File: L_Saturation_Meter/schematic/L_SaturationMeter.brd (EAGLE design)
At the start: 130 x 60 mm, 77 parts, among them IC1 LM317, IC4 LM358, SW1 DUR_10X, T1 IRF830, T2 BC847, T3 BC847, T4 BC847, T5 BC847, T6 IRF830, T7 IRF830, X1 I_SENSE_100x, X2 POWER_12V, X3 L_TEST_END, X4 I_SENSE_10x, X5 Synchro, X6 L_TEST_END

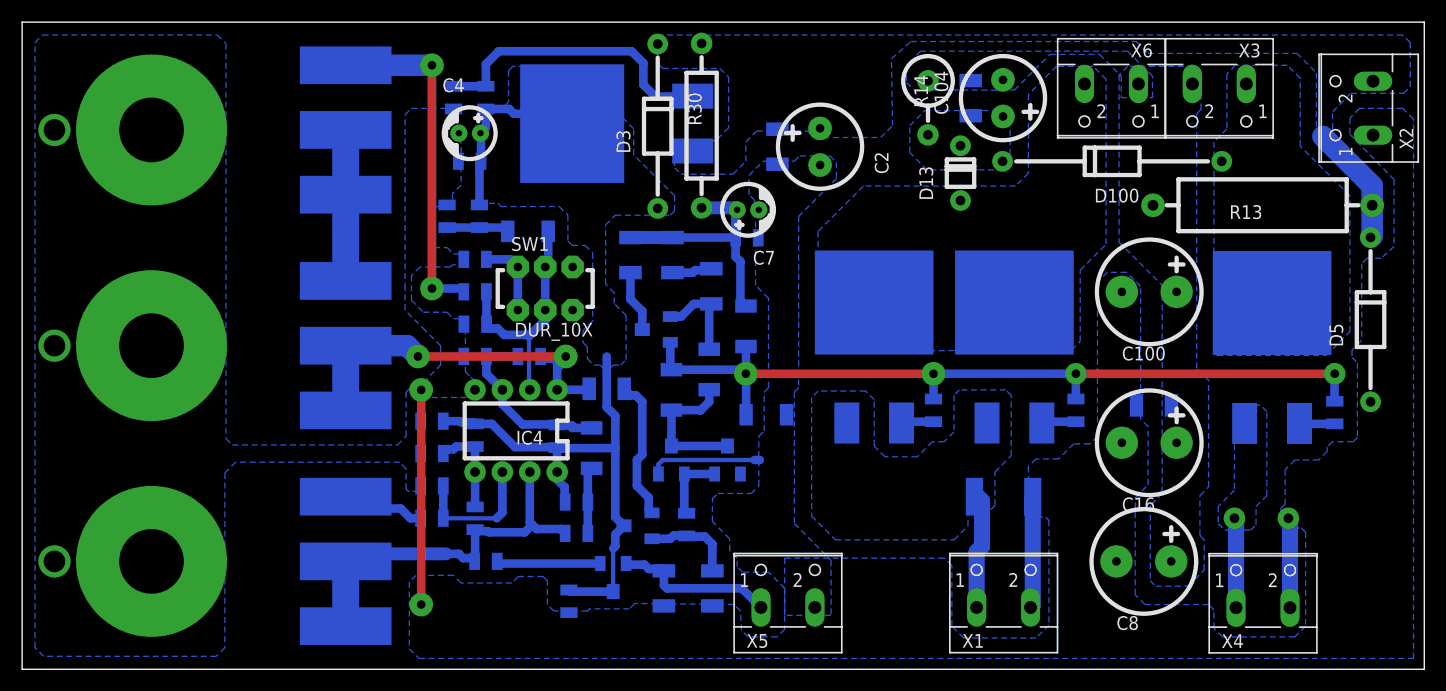
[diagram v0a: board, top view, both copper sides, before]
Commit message: L saturation meter. Routed
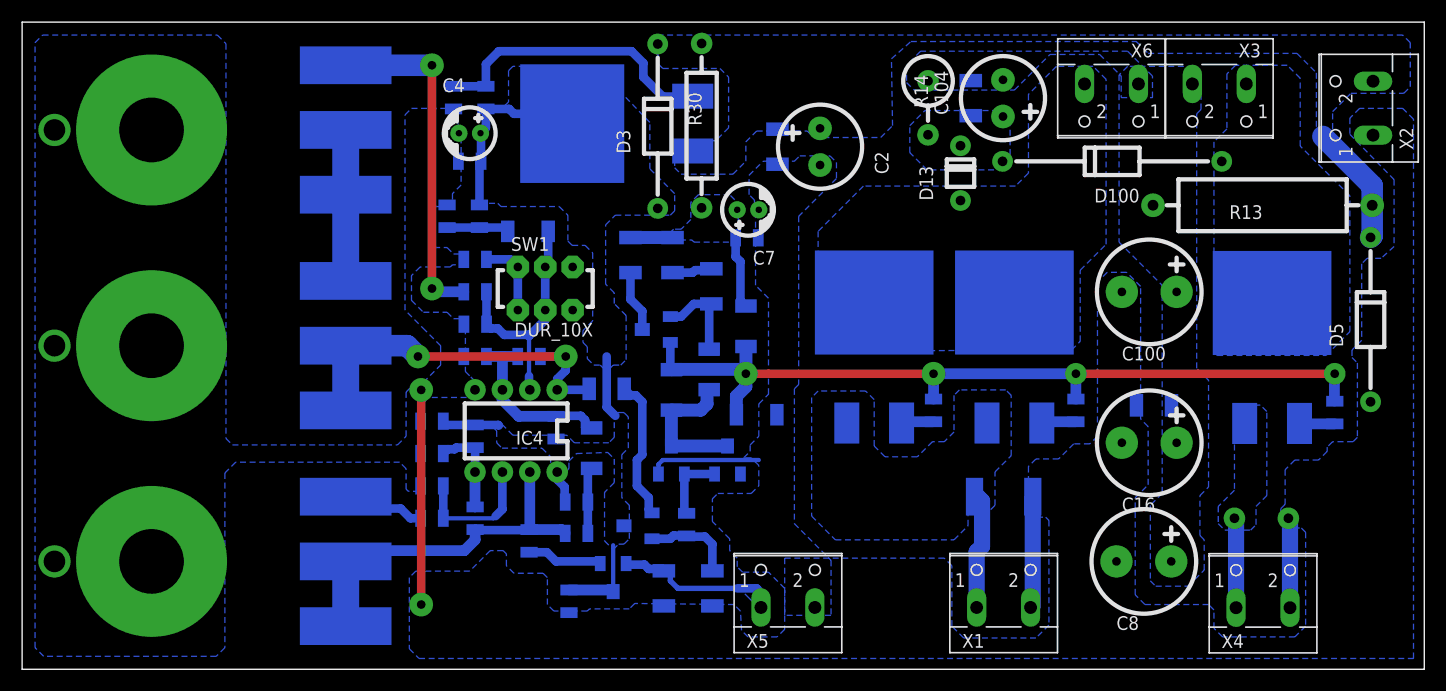
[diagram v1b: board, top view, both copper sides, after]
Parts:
- moved R18 4.43 mm to (47.0, 11.9), turned to 90 degrees
- moved D14 0.90 mm to (68.1, 23.6)
- moved R3 0.81 mm to (49.5, 22.4)
- moved R16 0.10 mm to (42.0, 21.6)
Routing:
- net +VCC: track 67.1 -> 40.7 mm
- net N$33: track 22.5 -> 10.6 mm
- net N$19: track 9.63 -> 7.03 mm
- net N$13: track 35.6 -> 33.7 mm
- net N$20: track 15.0 -> 14.2 mm
- net N$14: track 17.3 -> 16.8 mm
- added copper zone on layer 16, net N$20
- added copper zone on layer 16, net N$33

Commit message: L saturation meter. tiny fixes
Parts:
- R1: value 1K0 -> 5K6
- R19: value 510R -> 470R
- R2: value 3K0 -> 1K0
- R24: value 330R -> 470R

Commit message: L saturation meter. Final changes
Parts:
- R1: value 5K6 -> 4K7
- R13: value 1R0 -> 1R5
- R25, R26: value 510R -> 240R
- R27: value 20R -> 10R
- R6: value 1K0 -> 4K7
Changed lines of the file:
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@@
 <layer number="14" name="Route14" color="1" fill="6" visible="no" active="no"/>
 <layer number="15" name="Route15" color="4" fill="6" visible="no" active="no"/>
-<layer number="16" name="Bottom" color="1" fill="1" visible="no" active="yes"/>
+<layer number="16" name="Bottom" color="1" fill="1" visible="yes" active="yes"/>
 <layer number="17" name="Pads" color="2" fill="1" visible="yes" active="yes"/>
 <layer number="18" name="Vias" color="2" fill="1" visible="no" active="yes"/>
@@
 <attribute name="VALUE" x="71.69" y="26" size="1.27" layer="28" font="vector" ratio="20" rot="MR90"/>
 </element>
-<element name="R13" library="__MyCommonLib1" package="R_2.0W" value="1R0" x="115.01" y="43.02" smashed="yes" rot="R180">
+<element name="R13" library="__MyCommonLib1" package="R_2.0W" value="1R5" x="115.01" y="43.02" smashed="yes" rot="R180">
 <attribute name="NAME" x="115.01" y="43.02" size="1.27" layer="25" font="vector" ratio="20" rot="R180"/>
 <attribute name="VALUE" x="115.01" y="43.02" size="1.27" layer="27" font="vector" ratio="20" rot="R180"/>
@@
 <attribute name="VALUE" x="57.66" y="47.81" size="1.27" layer="27" font="vector" ratio="20" rot="R90"/>
 </element>
-<element name="R1" library="__MyCommonLib1" package="RSMD_0805" value="5K6" x="40" y="53" smashed="yes" rot="MR90">
+<element name="R1" library="__MyCommonLib1" package="RSMD_0805" value="4K7" x="40" y="53" smashed="yes" rot="MR90">
 <attribute name="NAME" x="40" y="53" size="1.27" layer="26" font="vector" ratio="20" rot="MR90"/>
 <attribute name="VALUE" x="36.9" y="51.3" size="1.27" layer="28" font="vector" ratio="20" rot="MR90"/>
@@
 <attribute name="VALUE" x="54.5" y="16.9" size="1.27" layer="28" font="vector" ratio="20" rot="MR90"/>
 </element>
-<element name="R6" library="__MyCommonLib1" package="RSMD_0805" value="1K0" x="51.4" y="15.5" smashed="yes" rot="MR180">
+<element name="R6" library="__MyCommonLib1" package="RSMD_0805" value="4K7" x="51.4" y="15.5" smashed="yes" rot="MR180">
 <attribute name="NAME" x="51.4" y="15.5" size="1.27" layer="26" font="vector" ratio="20" rot="MR180"/>
 <attribute name="VALUE" x="49.7" y="16" size="1.27" layer="28" font="vector" ratio="20" rot="MR180"/>
@@
 <attribute name="VALUE" x="68.8" y="26" size="1.27" layer="28" font="vector" ratio="20" rot="MR90"/>
 </element>
-<element name="R25" library="__MyCommonLib1" package="RSMD_1206_BIG_GAP" value="510R" x="63.9" y="35.5" smashed="yes" rot="MR270">
+<element name="R25" library="__MyCommonLib1" package="RSMD_1206_BIG_GAP" value="240R" x="63.9" y="35.5" smashed="yes" rot="MR270">
 <attribute name="NAME" x="63.9" y="35.5" size="1.27" layer="26" font="vector" ratio="20" rot="MR270"/>
 <attribute name="VALUE" x="64.6" y="37.6" size="1.27" layer="28" font="vector" ratio="20" rot="MR270"/>
 </element>
-<element name="R26" library="__MyCommonLib1" package="RSMD_1206_BIG_GAP" value="510R" x="60.3" y="38.4" smashed="yes" rot="MR270">
+<element name="R26" library="__MyCommonLib1" package="RSMD_1206_BIG_GAP" value="240R" x="60.3" y="38.4" smashed="yes" rot="MR270">
 <attribute name="NAME" x="60.3" y="38.4" size="1.27" layer="26" font="vector" ratio="20" rot="MR270"/>
 <attribute name="VALUE" x="60.4" y="41.7" size="1.27" layer="28" font="vector" ratio="20" rot="MR90"/>
 </element>
-<element name="R27" library="__MyCommonLib1" package="RSMD_1206_BIG_GAP" value="20R" x="56.4" y="38.4" smashed="yes" rot="MR270">
+<element name="R27" library="__MyCommonLib1" package="RSMD_1206_BIG_GAP" value="10R" x="56.4" y="38.4" smashed="yes" rot="MR270">
 <attribute name="NAME" x="56.4" y="38.4" size="1.27" layer="26" font="vector" ratio="20" rot="MR270"/>
 <attribute name="VALUE" x="55.9" y="41.9" size="1.27" layer="28" font="vector" ratio="20" rot="MR90"/>
